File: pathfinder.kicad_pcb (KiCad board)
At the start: 2 copper layers, 60.5 x 86 mm, 29 parts, among them SW1 SW_Push, SW2 SW_Push, SW3 SW_Push, SW4 SW_Push, SW5 SW_Push, SW6 SW_Push, SW7 SW_Push, SW8 SW_Push, SW9 SW_Push, U1 XIAO-RP2040-DIP, U2 OLED_0.91_128x32

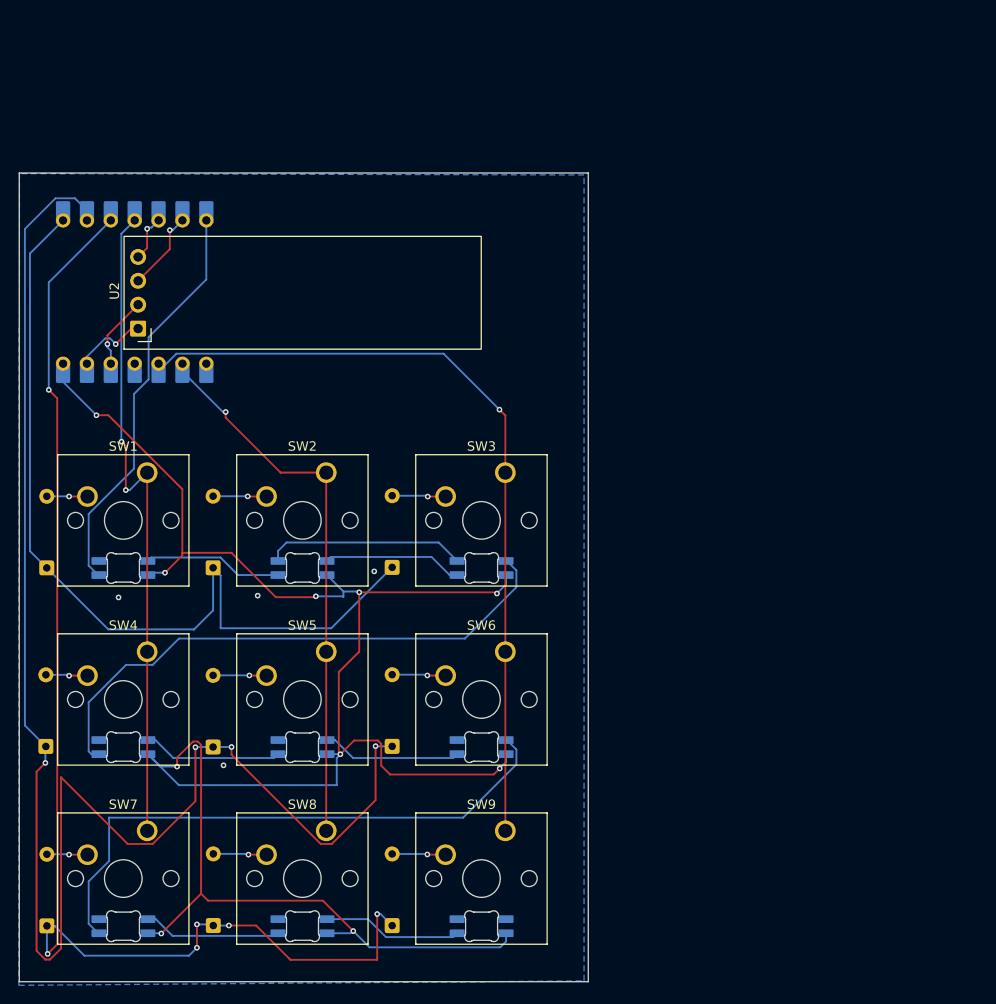
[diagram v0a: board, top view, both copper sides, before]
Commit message: fix
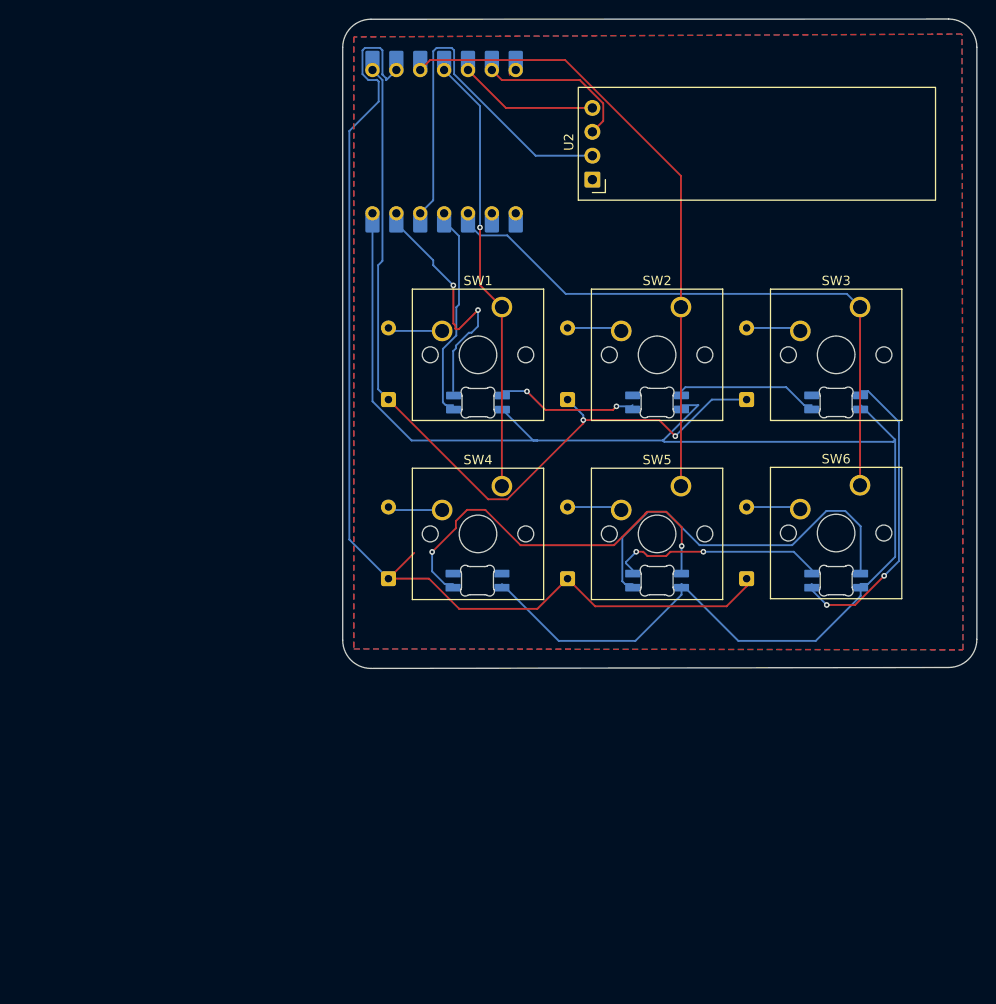
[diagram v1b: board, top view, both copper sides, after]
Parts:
- removed D13, D14, D15, D16, D17, D18: SK6812MINI-E, Hackclub Footprints:MX_SK6812MINI-E_REV
- removed SW7, SW8, SW9: SW_Push, Button_Switch_Keyboard:SW_Cherry_MX_1.00u_PCB
- D7, D8, D9: value D -> SK6812MINI-E; footprint Diode_THT:D_DO-35_SOD27_P7.62mm_Horizontal -> Hackclub Footprints:MX_SK6812MINI-E_REV; moved to F.Cu
- moved D9 76.9 mm to (175.8, 82.4), turned to 0 degrees
- moved D8 76.9 mm to (156.8, 82.4), turned to 0 degrees
- moved D7 76.1 mm to (137.7, 82.4), turned to 0 degrees
- moved D10 75.8 mm to (175.8, 101.3)
- moved U2 50.9 mm to (149.9, 63.8)
- moved D5 41.7 mm to (147.2, 106.2)
- moved D2 41.7 mm to (147.2, 87.2)
- moved D3 41.7 mm to (166.3, 87.2)
- moved D6 41.7 mm to (166.3, 106.2)
- moved SW6 41.7 mm to (175.8, 101.3)
- moved SW5 41.6 mm to (156.8, 101.4)
- moved SW1 41.6 mm to (137.7, 82.4)
- moved SW4 41.6 mm to (137.7, 101.4)
- moved SW3 41.6 mm to (175.8, 82.4)
- moved SW2 41.6 mm to (156.8, 82.4)
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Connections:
- D10 pad 1: VBUS -> 5V
- D10 pad 4: DIN1 -> Net-(D10-DIN)
- D11 pad 1: VBUS -> 5V
- D12 pad 1: VBUS -> 5V
- D12 pad 2: Net-(D12-DOUT) -> unconnected-(D12-DOUT-Pad2)
- D7 pad 1: ROW3 -> 5V
- D7 pad 2: Net-(D7-A) -> Net-(D7-DOUT)
- D8 pad 1: ROW3 -> 5V
- D8 pad 2: Net-(D8-A) -> Net-(D8-DOUT)
- D9 pad 1: ROW3 -> 5V
- D9 pad 2: Net-(D9-A) -> Net-(D10-DIN)
- U1 pad 11: unconnected-(U1-GPIO3/MOSI-Pad11)_1 -> Net-(D7-DIN)
- U1 pad 14: VBUS -> 5V
- U1 pad 3: ROW3 -> COL2
- U1 pad 7: DIN1 -> ENC_A
- U1 pad 8: unconnected-(U1-GPIO1/RX-Pad8)_1 -> ENC_B
- U1 pad 9: COL2 -> ENC_SW
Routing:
- net VBUS: track 209.0 -> 0.00 mm, vias 10 -> 0
- net 5V: track 0.00 -> 161.8 mm
- net ROW3: track 132.4 -> 0.00 mm, vias 6 -> 0
- net Net-(D15-DOUT): track 62.5 -> 0.00 mm
- net Net-(D12-DOUT): track 60.3 -> 0.00 mm
- net ROW2: track 167.6 -> 115.3 mm, vias 4 -> 0
- net DIN1: track 44.3 -> 0.00 mm
- net VCC: track 7.77 -> 41.1 mm, vias 1 -> 0
- net Net-(D10-DIN): track 0.00 -> 32.8 mm, vias 0 -> 2
- net Net-(D11-DOUT): track 14.8 -> 42.0 mm, vias 0 -> 2
- net Net-(D10-DOUT): track 14.8 -> 40.6 mm
- net COL1: track 70.6 -> 46.8 mm, vias 2 -> 1
- net Net-(D7-DIN): track 0.00 -> 21.9 mm
- net GND: track 29.2 -> 50.5 mm, vias 1 -> 4
- net COL3: track 84.6 -> 65.4 mm, vias 1 -> 0
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- added copper zone on F.Cu, net GND
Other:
- board size 60.5 x 86 mm -> 67.5 x 69.1 mm
